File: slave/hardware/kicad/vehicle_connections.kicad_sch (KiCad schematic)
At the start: 2 parts, among them J2 AMPSEAL_8, J3 AMPSEAL_23

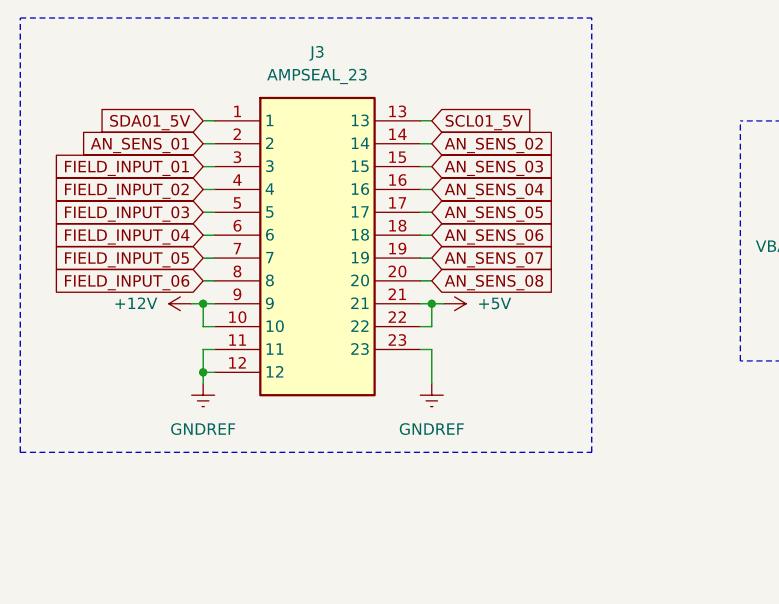
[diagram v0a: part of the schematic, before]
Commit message: feat(HW): begin PCB layout design
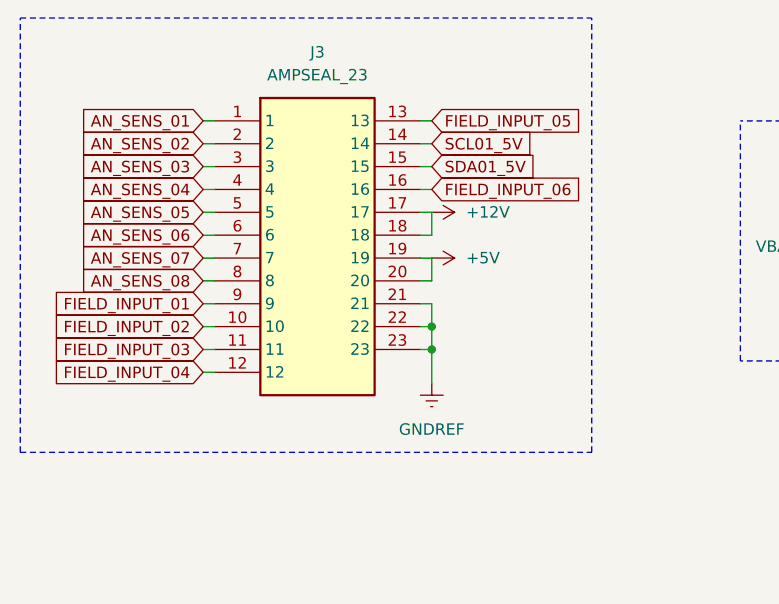
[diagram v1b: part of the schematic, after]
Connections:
- net +12V: now also J3.17, J3.18; no longer J3.10, J3.9
- net +5V: now also J3.19, J3.20; no longer J3.21, J3.22
- net AN_SENS_01: now also J3.1; no longer J3.2
- net AN_SENS_02: now also J3.2; no longer J3.14
- net AN_SENS_03: now also J3.3; no longer J3.15
- net AN_SENS_04: now also J3.4; no longer J3.16
- net AN_SENS_05: now also J3.5; no longer J3.17
- net AN_SENS_06: now also J3.6; no longer J3.18
- net AN_SENS_07: now also J3.7; no longer J3.19
- net AN_SENS_08: now also J3.8; no longer J3.20
- net FIELD_INPUT_01: now also J3.9; no longer J3.3
- net FIELD_INPUT_02: now also J3.10; no longer J3.4
- net FIELD_INPUT_03: now also J3.11; no longer J3.5
- net FIELD_INPUT_04: now also J3.12; no longer J3.6
- net FIELD_INPUT_05: now also J3.13; no longer J3.7
- net FIELD_INPUT_06: now also J3.16; no longer J3.8
- net GNDREF: now also J3.21, J3.22; no longer J3.11, J3.12
- net SCL01_5V: now also J3.14; no longer J3.13
- net SDA01_5V: now also J3.15; no longer J3.1
